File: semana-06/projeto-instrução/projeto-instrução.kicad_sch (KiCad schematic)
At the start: 8 parts, among them J2 Conn_01x02_Socket, K1 Relay_SPDT, Q1 BC107, U1 Pico

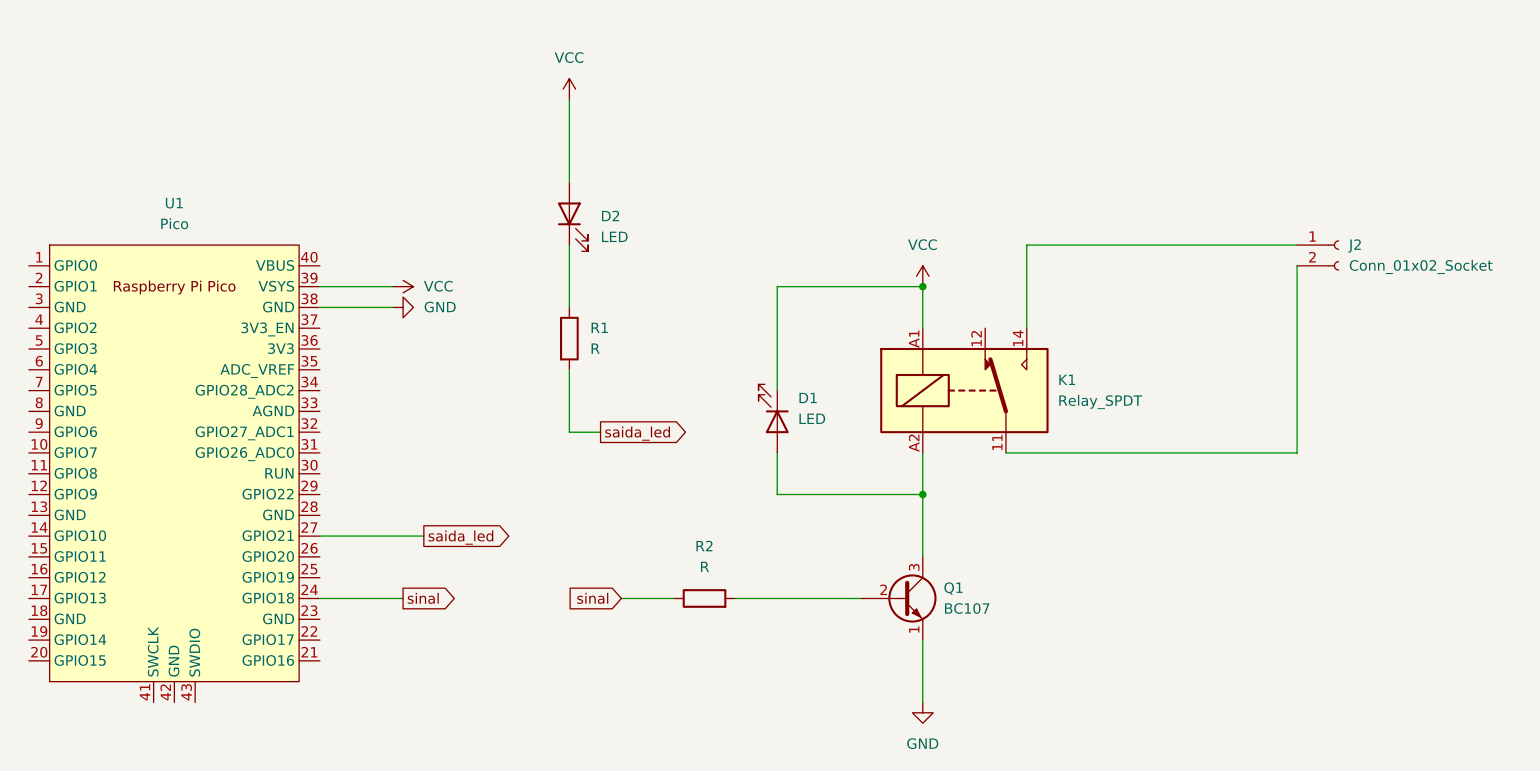
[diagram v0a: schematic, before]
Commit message: Ponderada Kicad
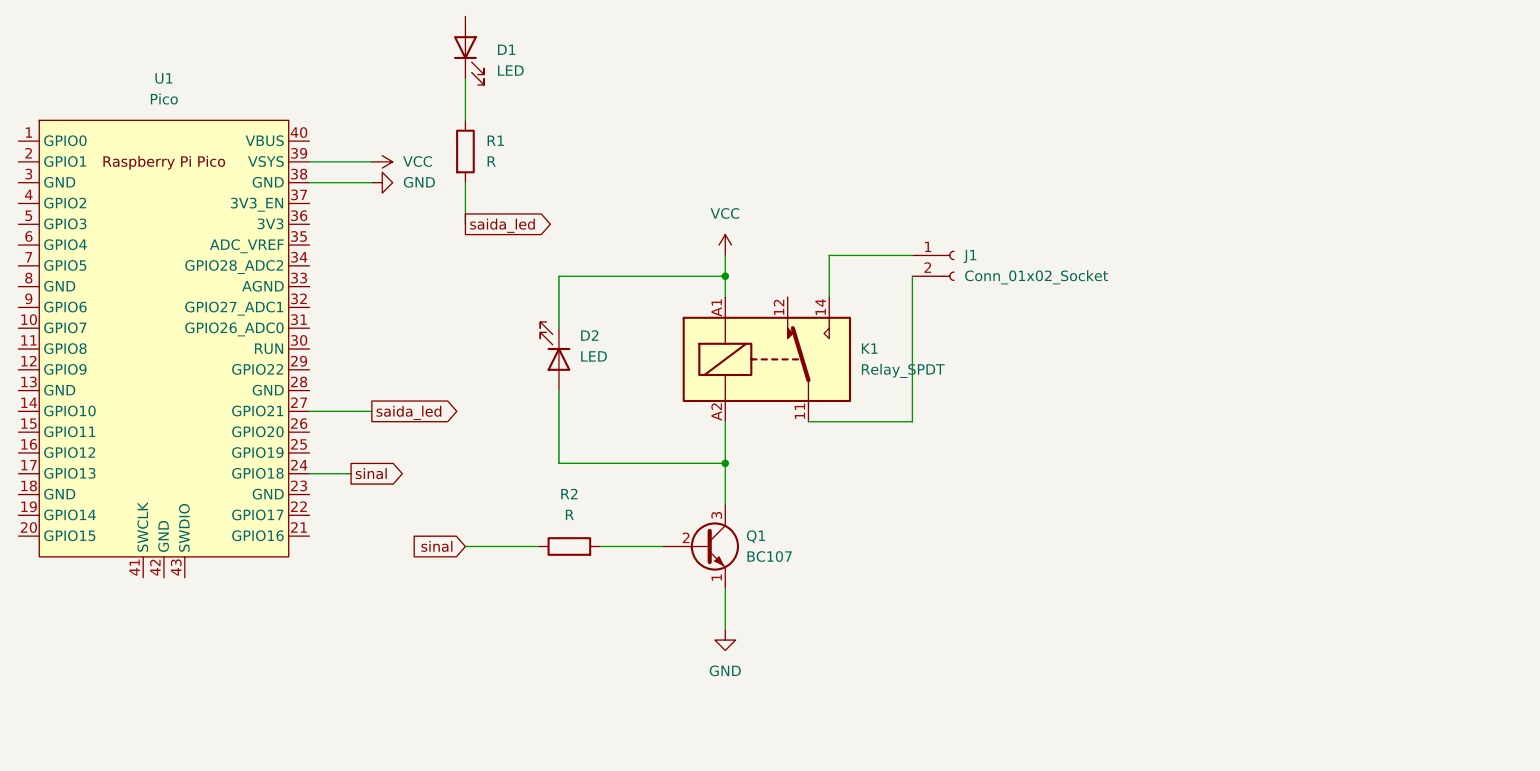
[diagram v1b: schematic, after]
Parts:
- removed J2: Conn_01x02_Socket, symbol Connector:Conn_01x02_Socket
- added J1: Conn_01x02_Socket, symbol Connector:Conn_01x02_Socket
- D1, D2: footprint LED_THT:LED_D5.0mm_Clear -> (none)
- K1: footprint Relay_THT:Relay_SPDT_Finder_40.51 -> (none)
- R1, R2: footprint Resistor_SMD:R_0805_2012Metric -> (none)
- U1: footprint MCU_RaspberryPi_and_Boards:RPi_Pico_SMD_TH -> RPi_Pico:RPi_Pico_SMD_TH
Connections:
- net VCC: now also D2.1 (K); no longer D1.1 (K), D2.2 (A)
- net at K1.A2, Q1.3 (C): now also D2.2 (A); no longer D1.2 (A)
- net at K1.14: now also J1.1 (Pin_1)
- net at K1.11: now also J1.2 (Pin_2)
- net at R1.1: now also D1.1 (K); no longer D2.1 (K)
